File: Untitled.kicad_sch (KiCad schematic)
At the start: 13 parts

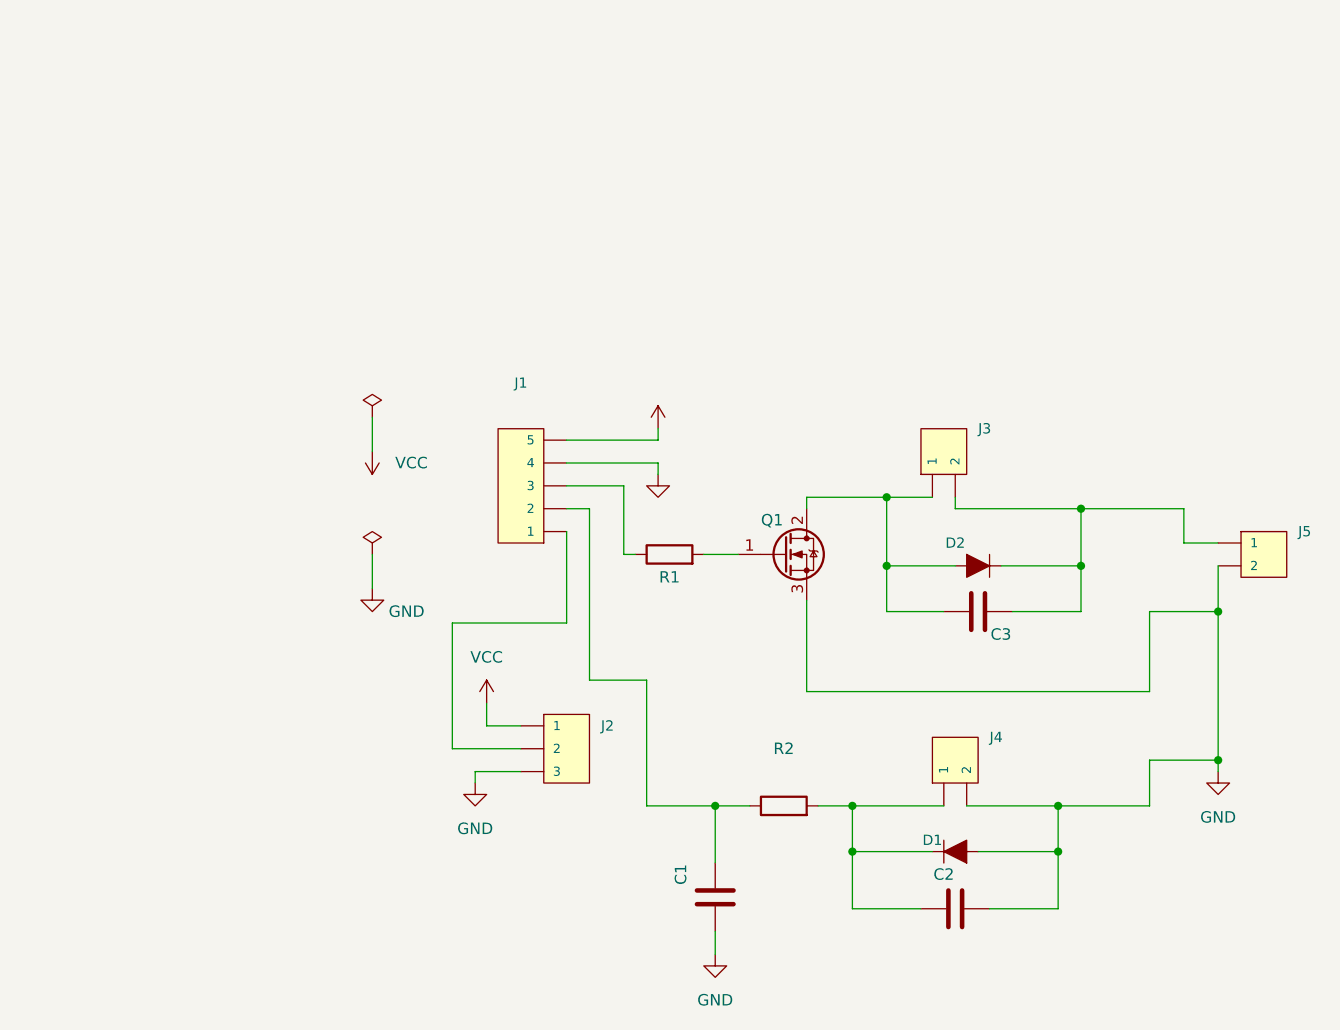
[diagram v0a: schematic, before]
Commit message: add images
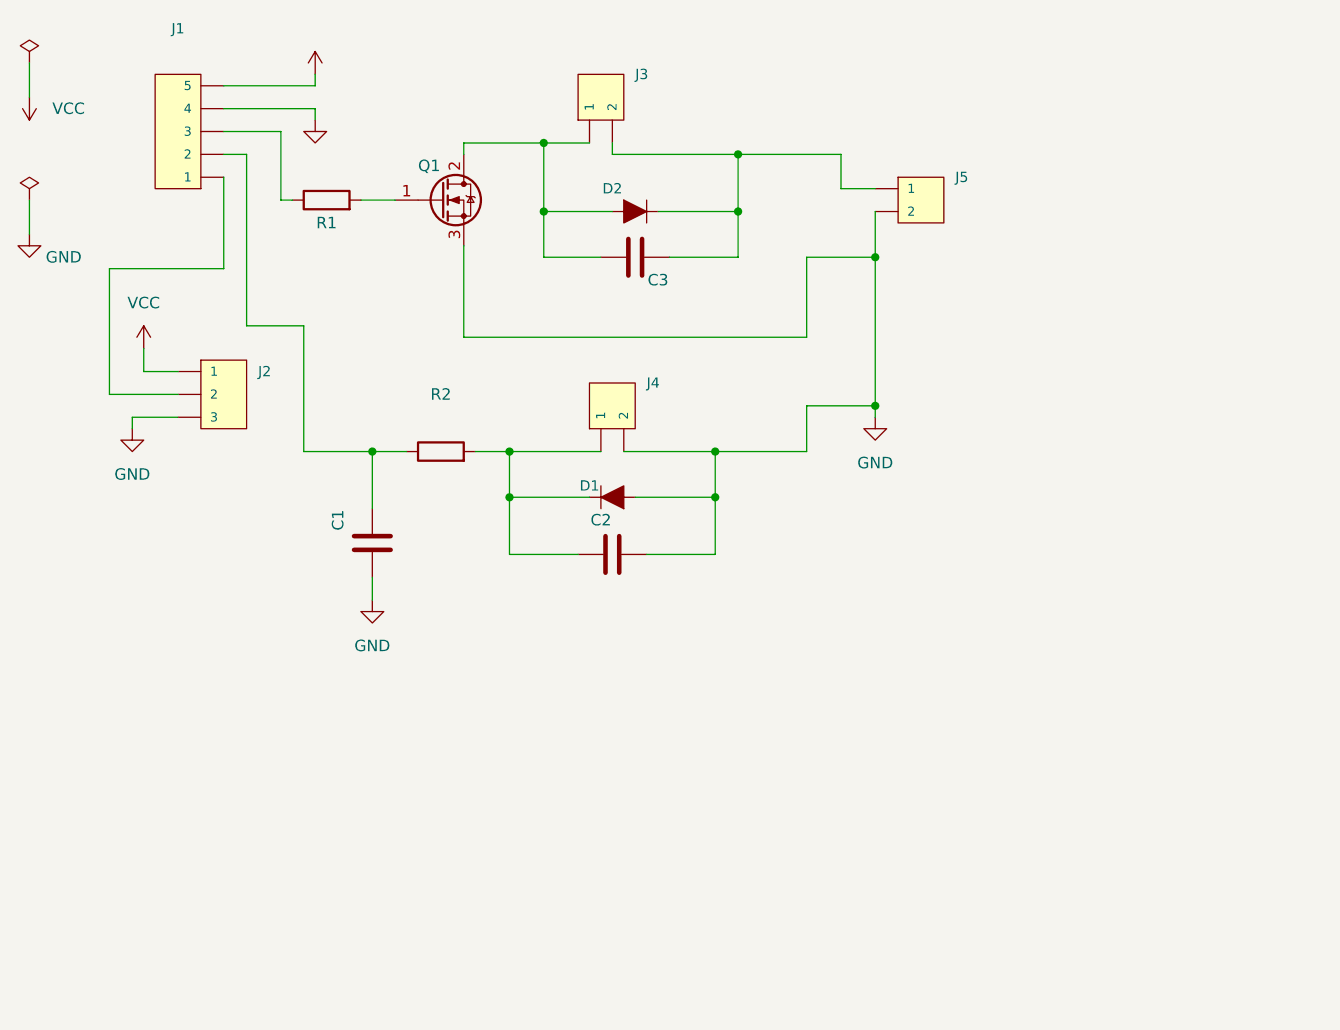
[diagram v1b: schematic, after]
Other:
- title: (none) -> Test PCB
- moved on the sheet: C1, C2, C3, D1, D2, J1, J2, J3, J4, J5, Q1, R1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
